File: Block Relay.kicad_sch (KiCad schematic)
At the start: 25 parts, among them J14 Screw_Terminal_01x02, J15 Screw_Terminal_01x02, J16 Screw_Terminal_01x02, J17 Screw_Terminal_01x02, J18 Screw_Terminal_01x02, K10 SRD-05VDC-SL-C, K5 SRD-05VDC-SL-C, K7 SRD-05VDC-SL-C, K8 SRD-05VDC-SL-C, K9 SRD-05VDC-SL-C, Q10 S8050, Q6 S8050, Q7 S8050, Q8 S8050, Q9 S8050

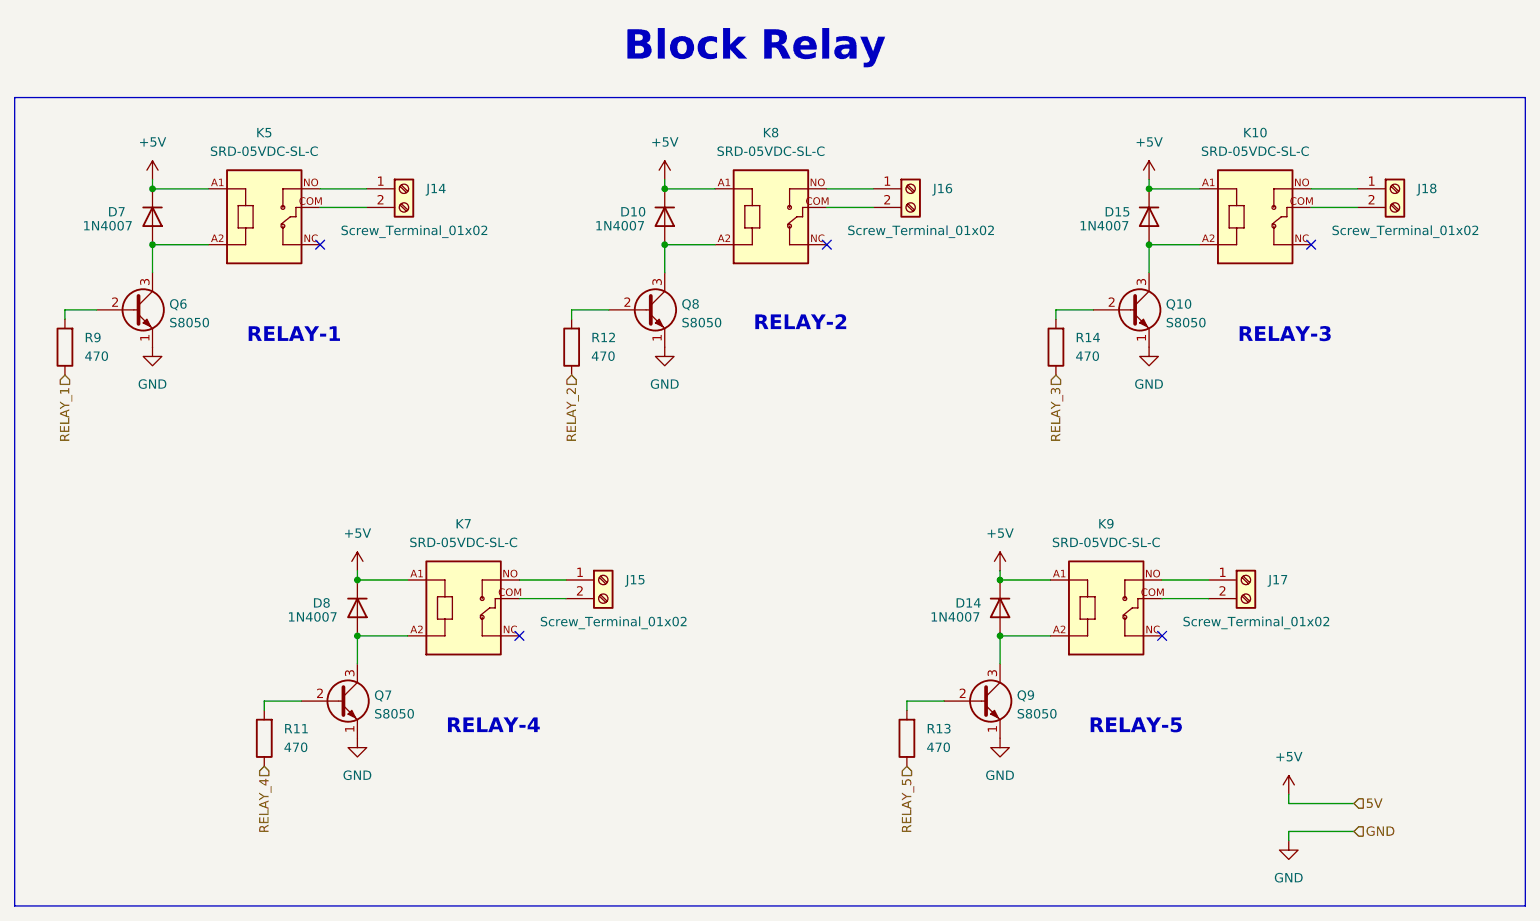
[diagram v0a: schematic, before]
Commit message: refactored project and fix some bugs
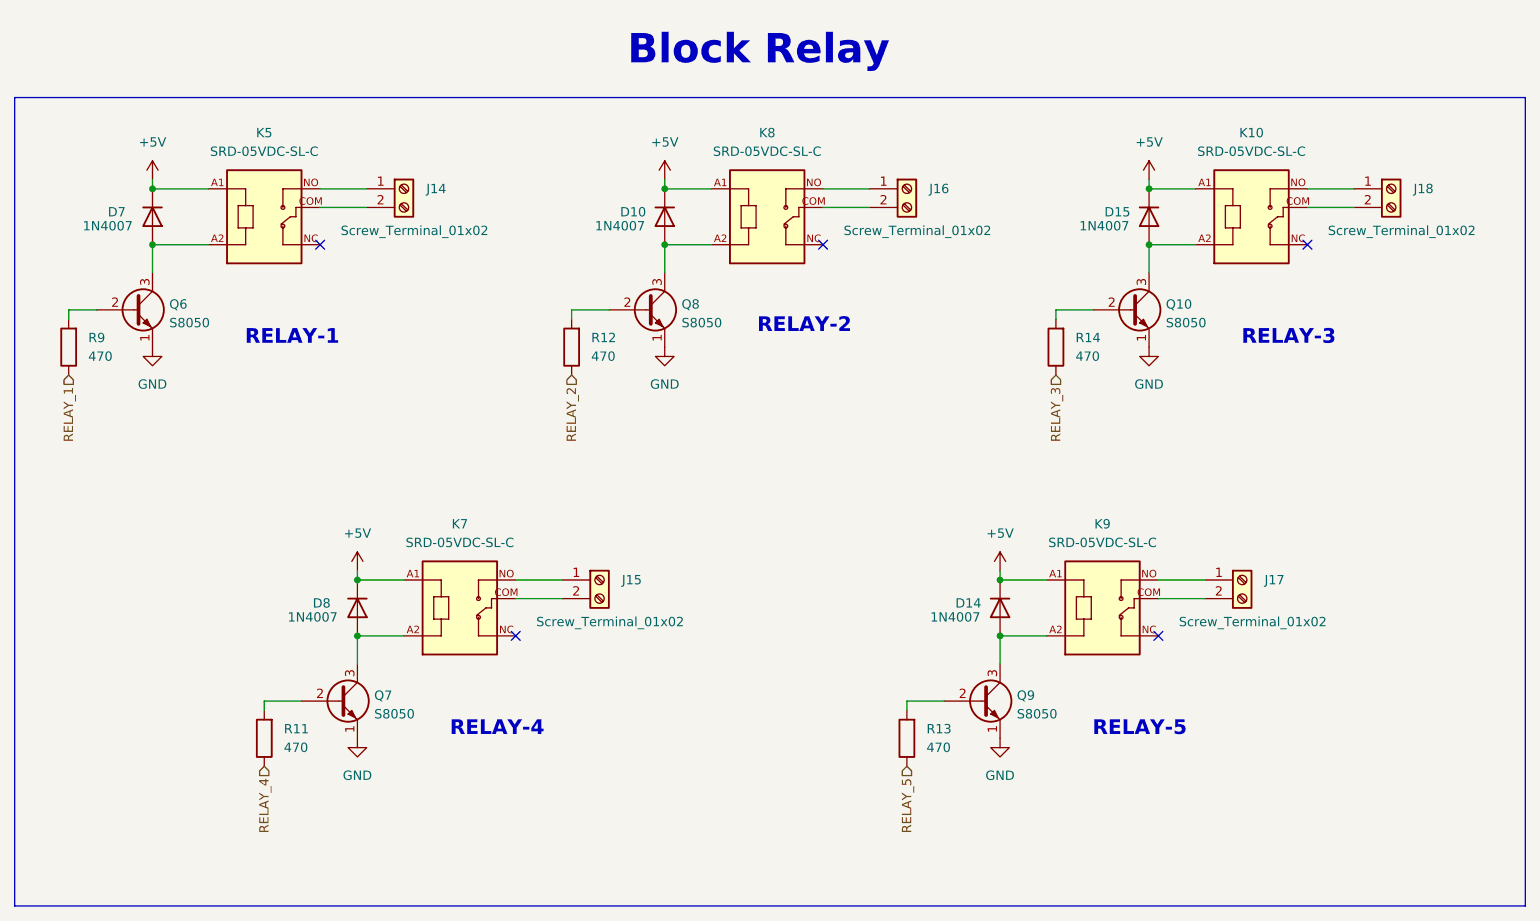
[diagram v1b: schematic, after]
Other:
- moved on the sheet: J15, J16, J17, J18, K10, K7, K8, K9, R9
